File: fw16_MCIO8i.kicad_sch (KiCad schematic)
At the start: 12 parts

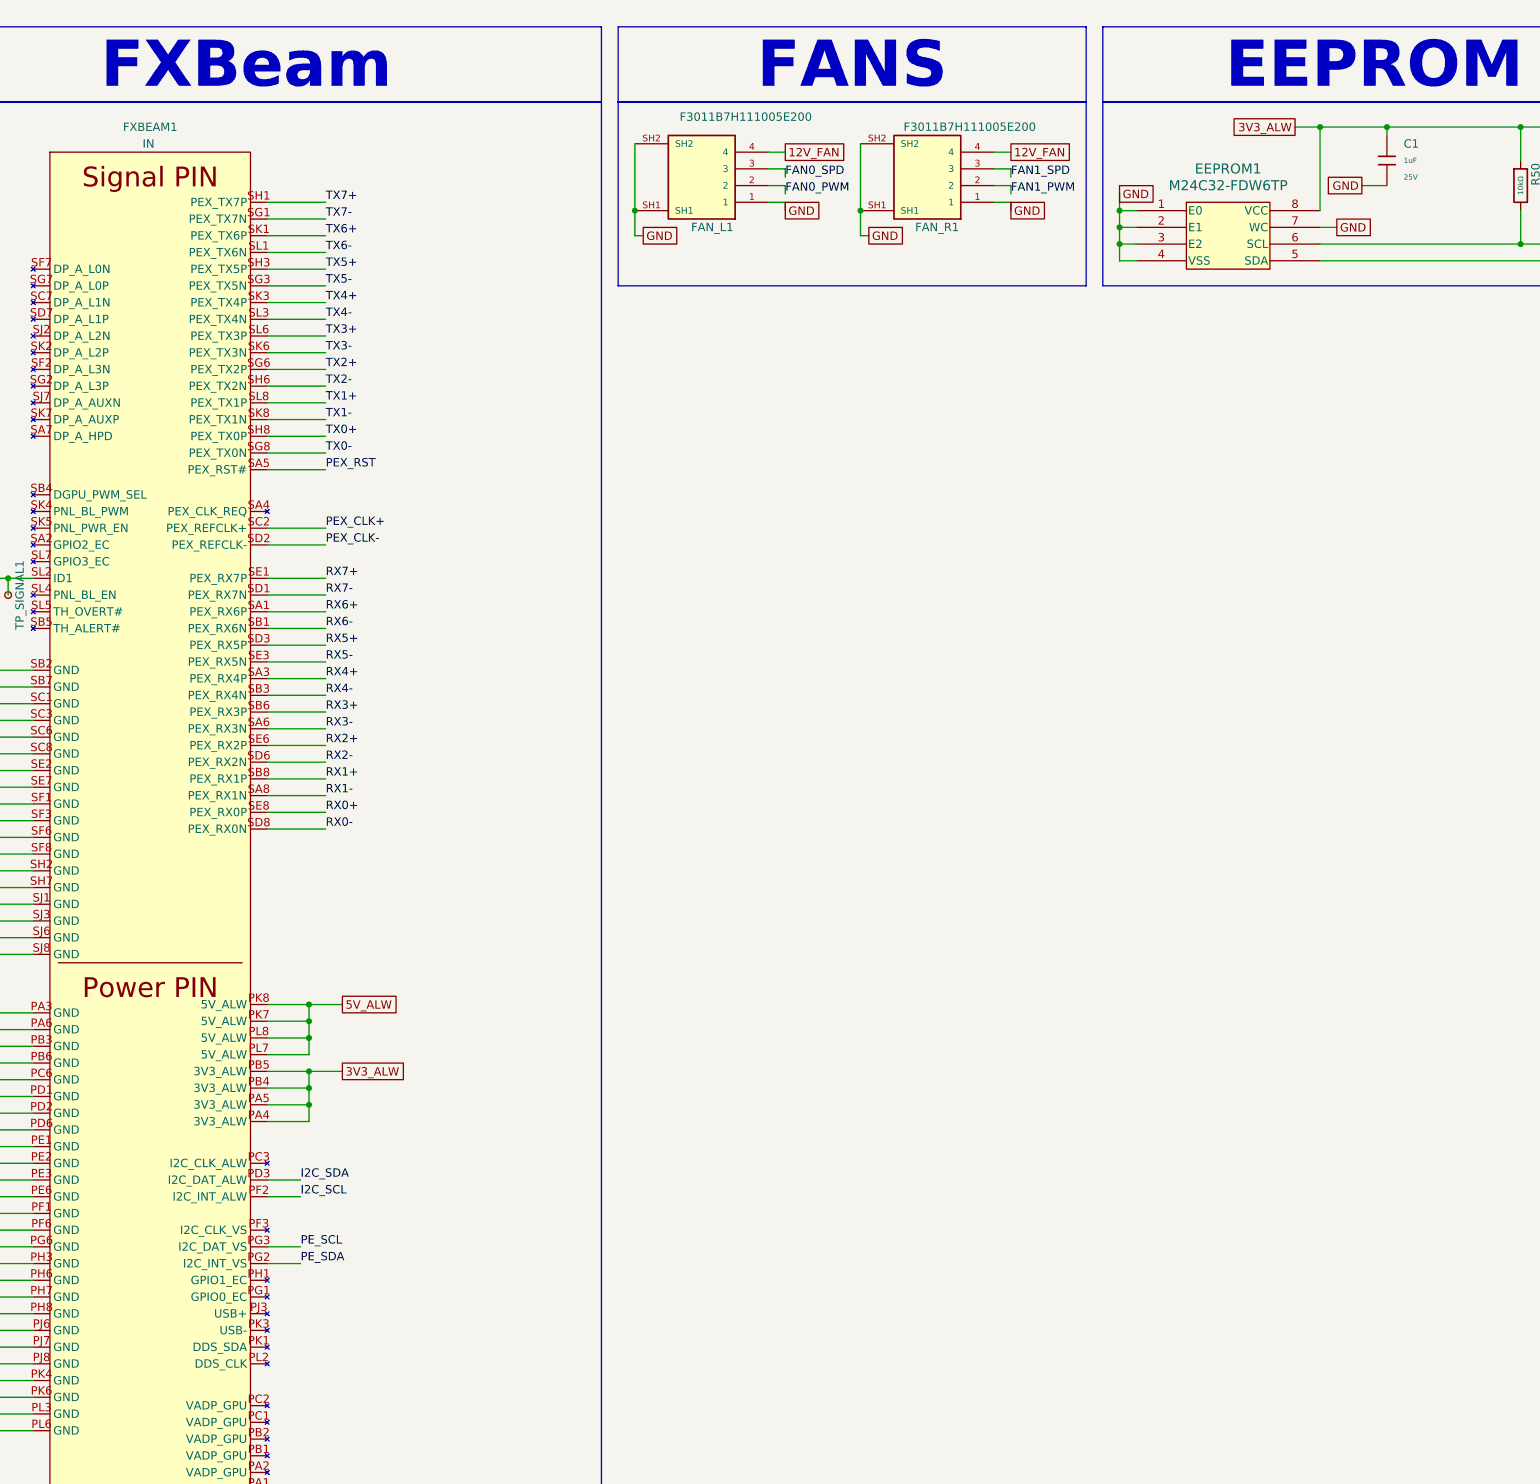
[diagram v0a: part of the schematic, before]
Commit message: New routing
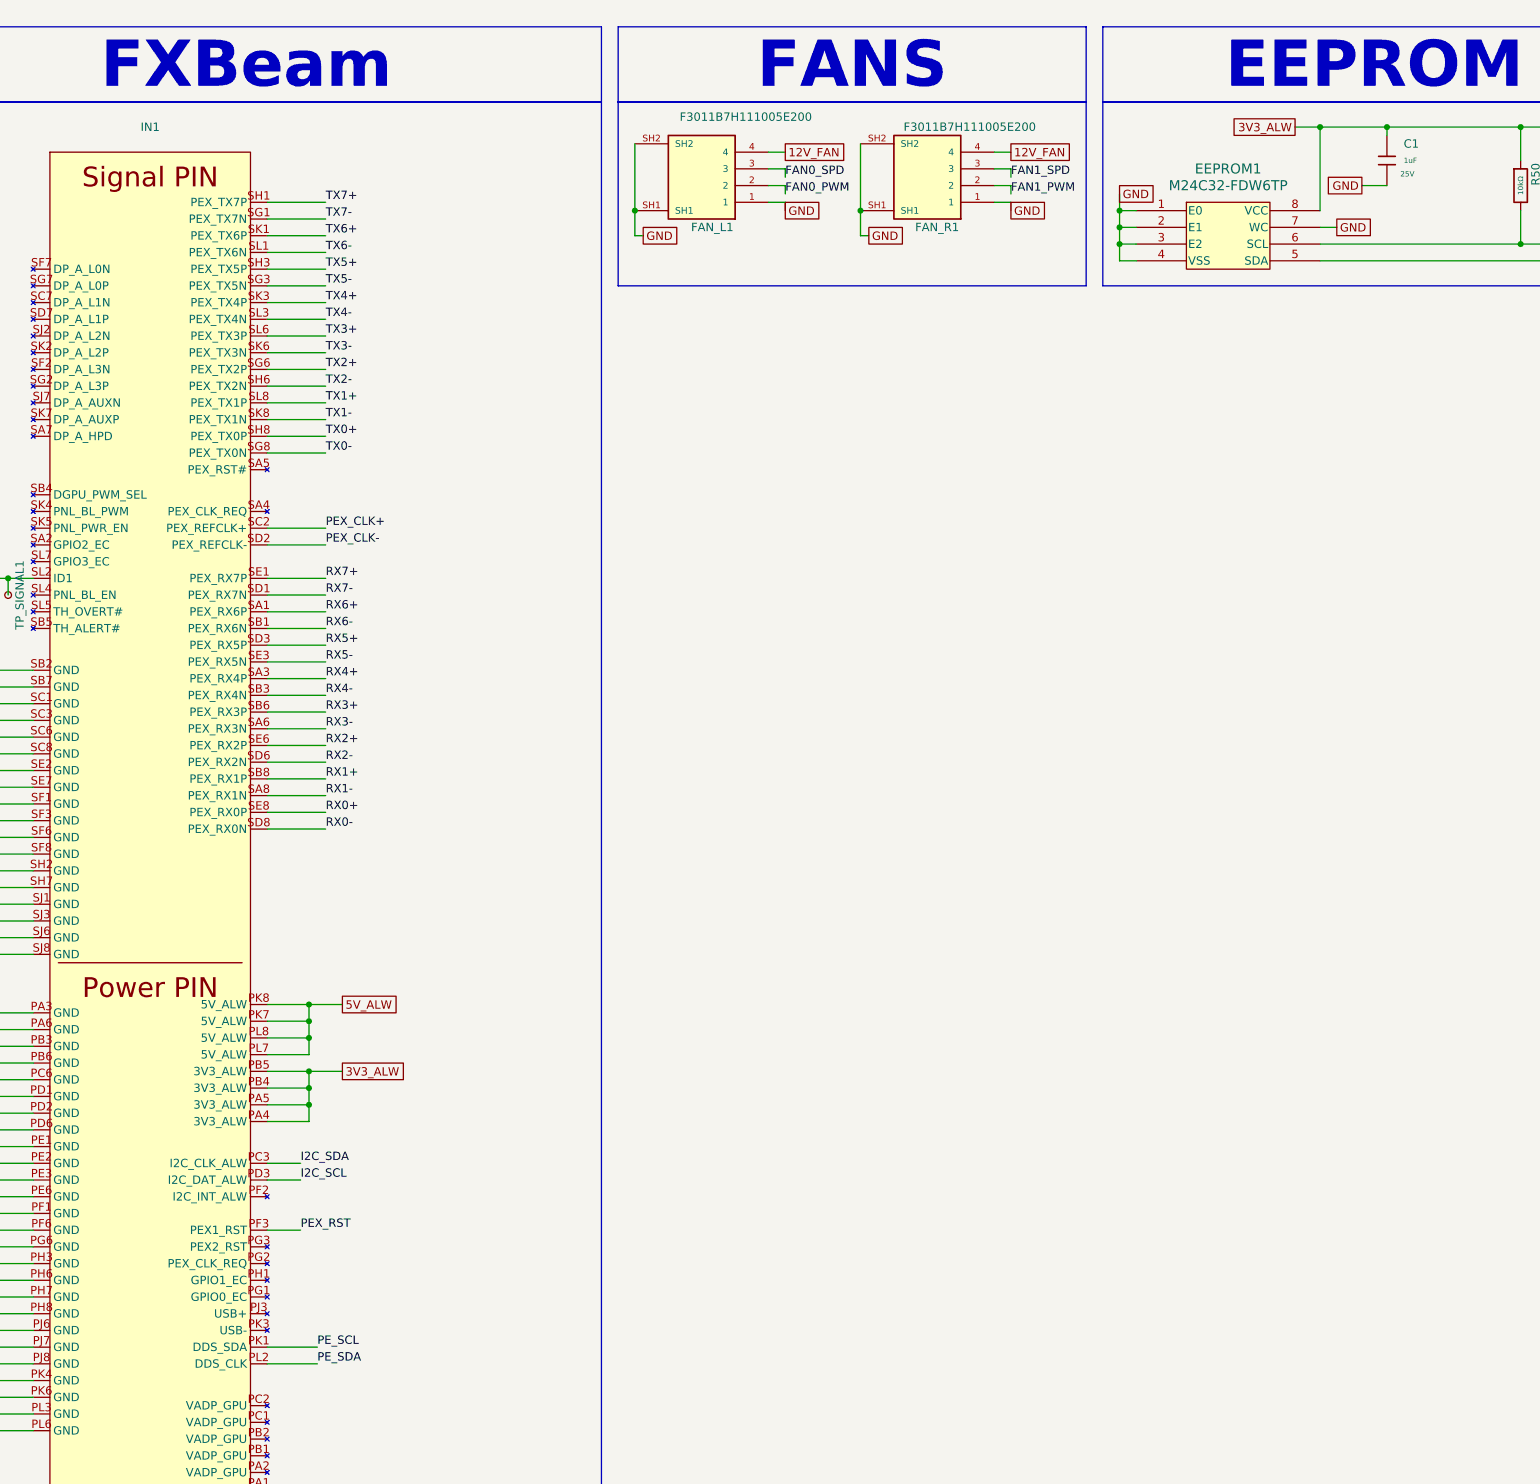
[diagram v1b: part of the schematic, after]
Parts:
- C1: MPN CL05A105KA5NQNC -> (none); PROD_ID CAP-25565 -> (none); Voltage 16V -> (none)
- EEPROM1: MPN M24C32-FDW6TP -> (none); now in the parts list
- IN1: renamed from FXBEAM1; value IN -> FXBEAM
- R1, R2: MPN 0402WGF3303TCE -> (none); PROD_ID RES-15407 -> (none)
- R50, R51: MPN 0402WGF1002TCE -> (none); PROD_ID RES-25567 -> (none)
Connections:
- net I2C_SCL: now also IN1.PD3 (I2C_DAT_ALW); no longer IN1.PF2 (I2C_INT_ALW)
- net I2C_SDA: now also IN1.PC3 (I2C_CLK_ALW); no longer IN1.PD3 (I2C_DAT_ALW)
- net PEX_RST: now also IN1.PF3 (PEX1_RST); no longer IN1.SA5 (PEX_RST#)
- net PE_SCL: now also IN1.PK1 (DDS_SDA); no longer IN1.PG3 (I2C_DAT_VS)
- net PE_SDA: now also IN1.PL2 (DDS_CLK); no longer IN1.PG2 (I2C_INT_VS)
